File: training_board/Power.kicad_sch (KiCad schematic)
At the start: 6 parts, among them U1 AP63203WU

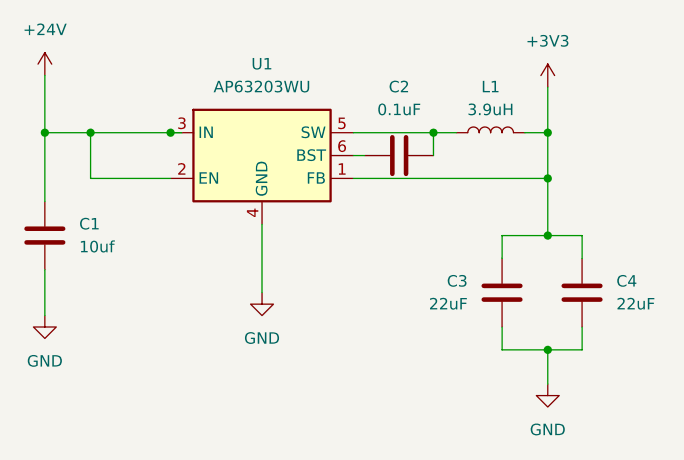
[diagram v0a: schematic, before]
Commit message: Cleaned up a bit
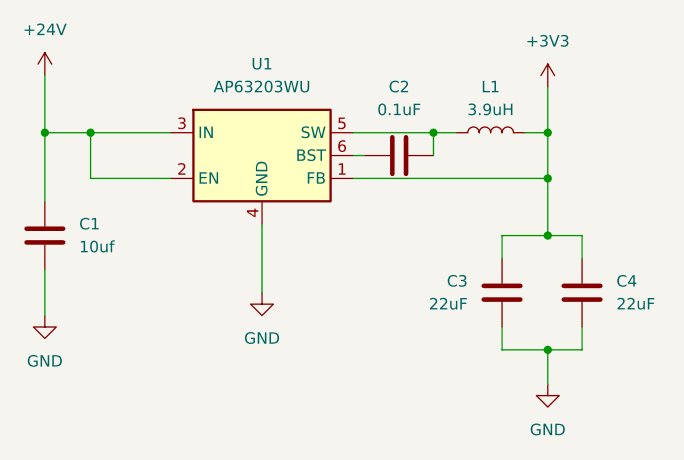
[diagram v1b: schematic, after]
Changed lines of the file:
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@@
 	(paper "A4")
 	(junction
+		(at 114.3 62.23)
+		(diameter 0)
+		(color 0 0 0 0)
+	)
+	(junction
 		(at 165.1 73.66)
 		(diameter 0)
@@
 	)
 	(junction
-		(at 114.3 62.23)
-		(diameter 0)
-		(color 0 0 0 0)
-	)
-	(junction
-		(at 123.19 62.23)
-		(diameter 0)
-		(color 0 0 0 0)
-	)
-	(junction
 		(at 165.1 67.31)
 		(diameter 0)
@@
 	(wire
 		(pts
-			(xy 124.46 62.23) (xy 123.19 62.23)
-		)
-		(stroke
-			(width 0)
-			(type default)
-		)
-	)
-	(wire
-		(pts
 			(xy 160.02 73.66) (xy 165.1 73.66)
 		)
@@
 	(wire
 		(pts
+			(xy 114.3 62.23) (xy 123.19 62.23)
+		)
+		(stroke
+			(width 0)
+			(type default)
+		)
+	)
+	(wire
+		(pts
 			(xy 160.02 86.36) (xy 160.02 83.82)
 		)
@@
 		)
 		(stroke
-			(width 0)
-			(type default)
-		)
-	)
-	(wire
-		(pts
-			(xy 123.19 62.23) (xy 114.3 62.23)
-		)
-		(stroke
